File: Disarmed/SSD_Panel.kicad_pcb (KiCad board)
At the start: 2 copper layers, 181.6 x 193 mm, 15 parts, among them J1 Conn_02x04_Counter_Clockwise, U1 MAX7219, U2 MCP41010, U3 MAX7219, U4 MAX7219, U5 MAX7219

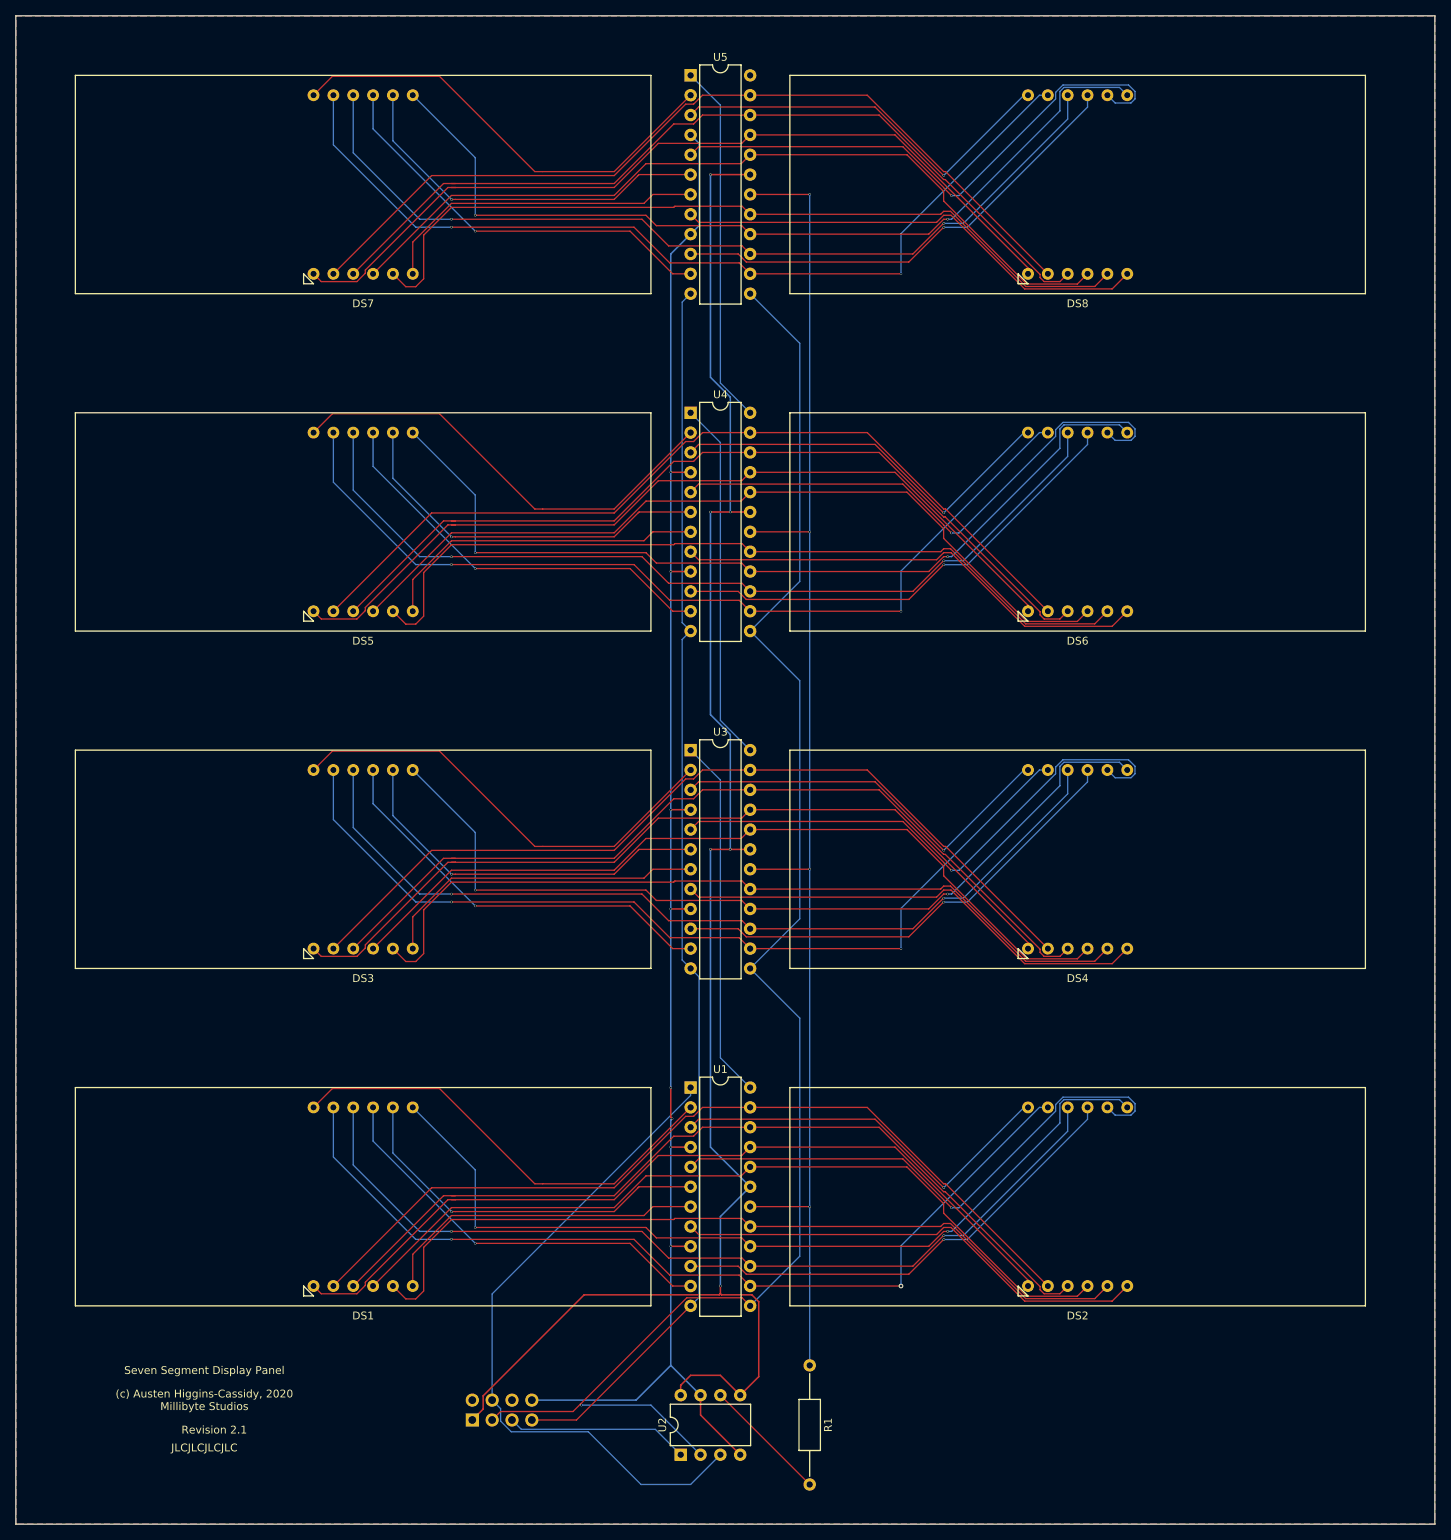
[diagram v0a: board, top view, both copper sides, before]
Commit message: Add new boards
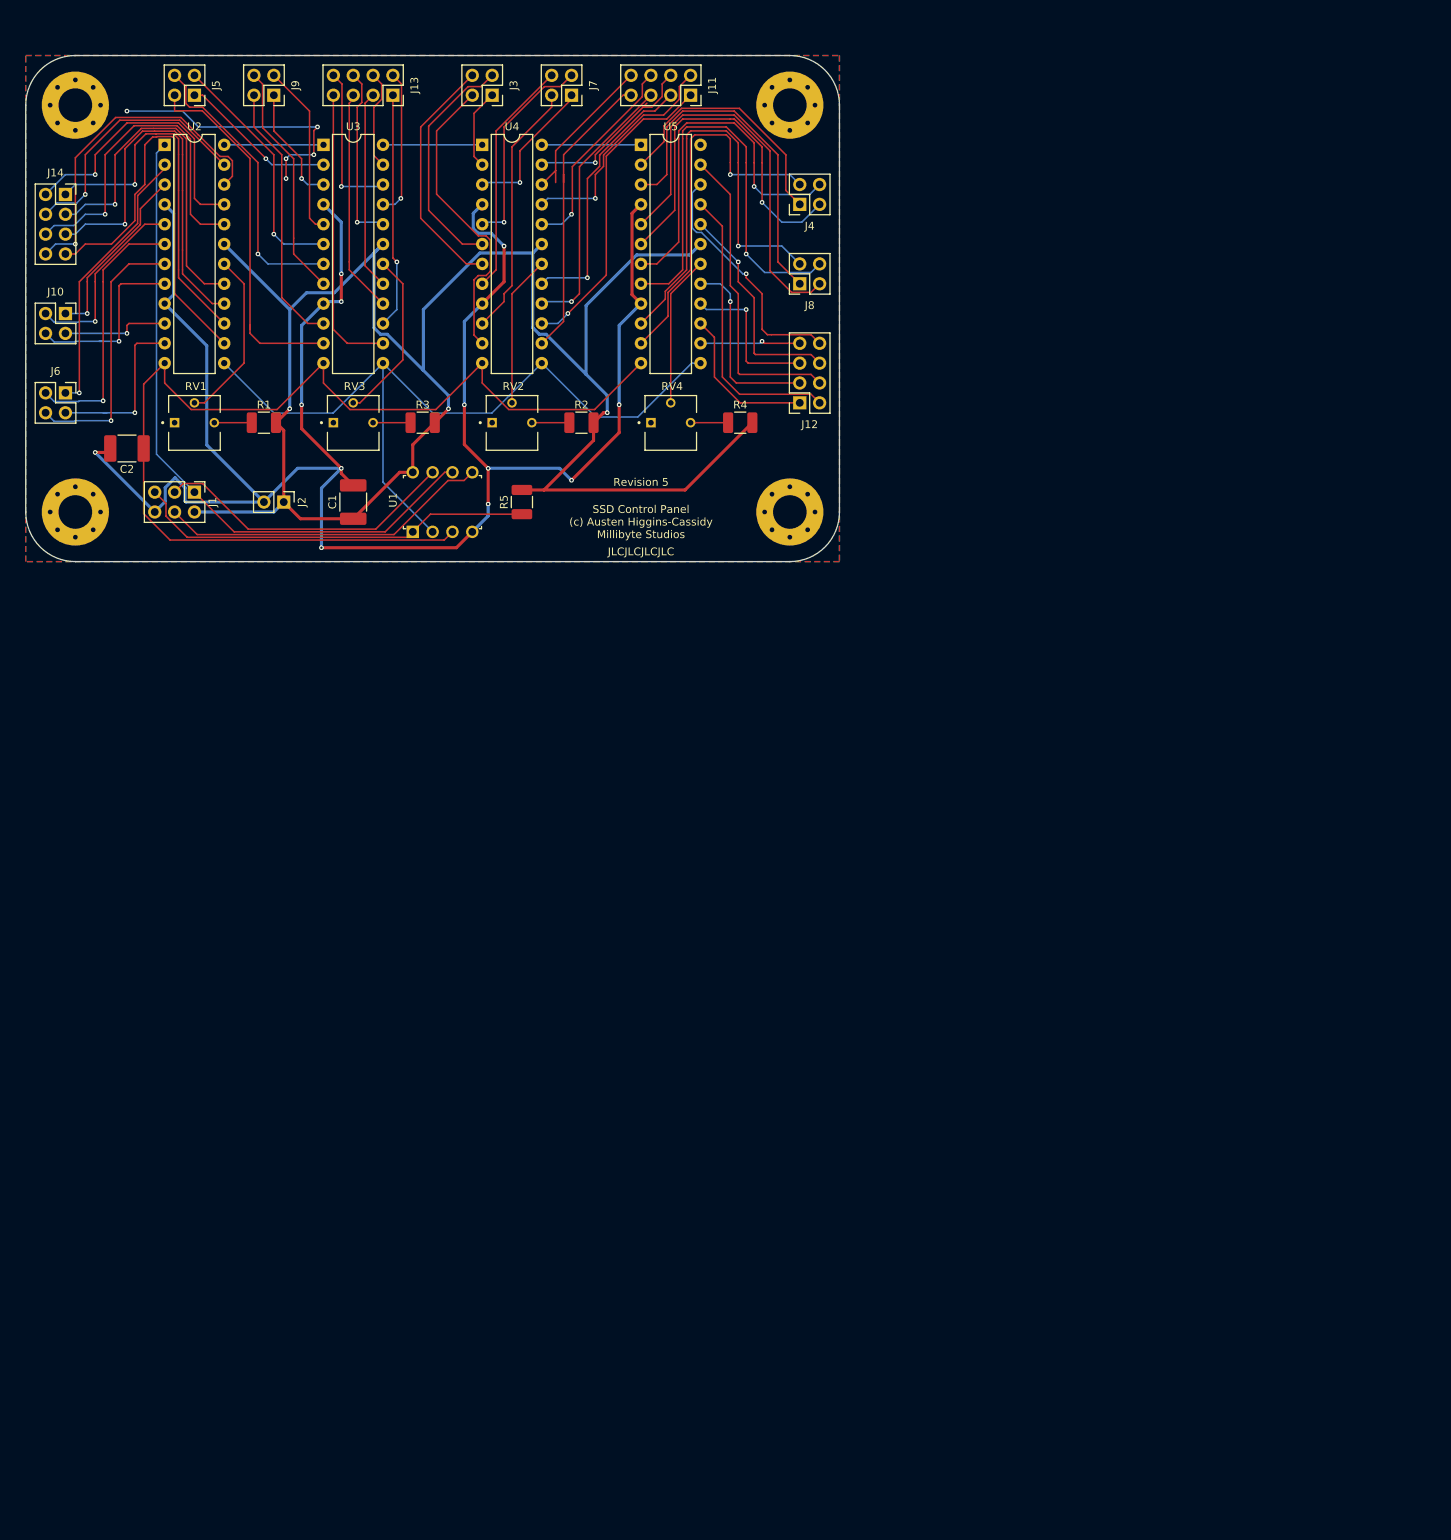
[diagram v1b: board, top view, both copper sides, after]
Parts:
- removed DS1, DS2, DS3, DS4, DS5, DS6, DS7, DS8: D8014CD, Disarmed:D8041CD
- added C1: 0.1uF, Capacitor_SMD:C_1812_4532Metric_Pad1.57x3.40mm_HandSolder, F.Cu at (57.1, 74.3)
- added C2: 10uF, Capacitor_SMD:C_1812_4532Metric_Pad1.57x3.40mm_HandSolder, F.Cu at (28.2, 67.4)
- added J10: Conn_02x02_Odd_Even, Connector_PinSocket_2.54mm:PinSocket_2x02_P2.54mm_Vertical, F.Cu at (20.3, 50.2)
- added J11: Conn_02x04_Odd_Even, Connector_PinSocket_2.54mm:PinSocket_2x04_P2.54mm_Vertical, F.Cu at (100.3, 22.2)
- added J12: Conn_02x04_Odd_Even, Connector_PinSocket_2.54mm:PinSocket_2x04_P2.54mm_Vertical, F.Cu at (114.3, 61.6)
- added J13: Conn_02x04_Odd_Even, Connector_PinSocket_2.54mm:PinSocket_2x04_P2.54mm_Vertical, F.Cu at (62.2, 22.2)
- added J14: Conn_02x04_Odd_Even, Connector_PinSocket_2.54mm:PinSocket_2x04_P2.54mm_Vertical, F.Cu at (20.3, 34.9)
- added J2: Conn_01x02_Male, Connector_PinHeader_2.54mm:PinHeader_1x02_P2.54mm_Vertical, F.Cu at (48.3, 74.3)
- added J3: Conn_02x02_Odd_Even, Connector_PinSocket_2.54mm:PinSocket_2x02_P2.54mm_Vertical, F.Cu at (74.9, 22.2)
- added J4: Conn_02x02_Odd_Even, Connector_PinSocket_2.54mm:PinSocket_2x02_P2.54mm_Vertical, F.Cu at (114.3, 36.2)
- added J5: Conn_02x02_Odd_Even, Connector_PinSocket_2.54mm:PinSocket_2x02_P2.54mm_Vertical, F.Cu at (36.8, 22.2)
- added J6: Conn_02x02_Odd_Even, Connector_PinSocket_2.54mm:PinSocket_2x02_P2.54mm_Vertical, F.Cu at (20.3, 60.3)
- added J7: Conn_02x02_Odd_Even, Connector_PinSocket_2.54mm:PinSocket_2x02_P2.54mm_Vertical, F.Cu at (85.1, 22.2)
- added J8: Conn_02x02_Odd_Even, Connector_PinSocket_2.54mm:PinSocket_2x02_P2.54mm_Vertical, F.Cu at (114.3, 46.4)
- added J9: Conn_02x02_Odd_Even, Connector_PinSocket_2.54mm:PinSocket_2x02_P2.54mm_Vertical, F.Cu at (47.0, 22.2)
- added R2: RMIN (2K), Resistor_SMD:R_1210_3225Metric_Pad1.30x2.65mm_HandSolder, F.Cu at (86.4, 64.1)
- added R3: RMIN (2K), Resistor_SMD:R_1210_3225Metric_Pad1.30x2.65mm_HandSolder, F.Cu at (66.0, 64.1)
- added R4: RMIN (2K), Resistor_SMD:R_1210_3225Metric_Pad1.30x2.65mm_HandSolder, F.Cu at (106.7, 64.1)
- added R5: 10K, Resistor_SMD:R_1210_3225Metric_Pad1.30x2.65mm_HandSolder, F.Cu at (78.7, 74.3)
- added REF**: MountingHole_4.3mm_M4_Pad_Via, Disarmed:MountingHole_4.3mm_M4_Pad_Via, F.Cu at (113.0, 23.5)
- added REF**: MountingHole_4.3mm_M4_Pad_Via, Disarmed:MountingHole_4.3mm_M4_Pad_Via, F.Cu at (113.0, 75.6)
- added REF**: MountingHole_4.3mm_M4_Pad_Via, Disarmed:MountingHole_4.3mm_M4_Pad_Via, F.Cu at (21.6, 75.6)
- added REF**: MountingHole_4.3mm_M4_Pad_Via, Disarmed:MountingHole_4.3mm_M4_Pad_Via, F.Cu at (21.6, 23.5)
- added RV1: R_POT, 3362P-1-103LF:TRIM_3362P-1-103LF, F.Cu at (36.8, 64.1)
- added RV2: R_POT, 3362P-1-103LF:TRIM_3362P-1-103LF, F.Cu at (77.5, 64.1)
- added RV3: R_POT, 3362P-1-103LF:TRIM_3362P-1-103LF, F.Cu at (57.1, 64.1)
- added RV4: R_POT, 3362P-1-103LF:TRIM_3362P-1-103LF, F.Cu at (97.8, 64.1)
- J1: value Conn_02x04_Counter_Clockwise -> Conn_02x03_Odd_Even; footprint Connector_PinSocket_2.54mm:PinSocket_2x04_P2.54mm_Vertical -> Connector_PinHeader_2.54mm:PinHeader_2x03_P2.54mm_Vertical; moved to F.Cu
- R1: value 2k -> RMIN (2K); footprint Resistor_THT:R_Axial_DIN0207_L6.3mm_D2.5mm_P15.24mm_Horizontal -> Resistor_SMD:R_1210_3225Metric_Pad1.30x2.65mm_HandSolder
- U1: value MAX7219 -> ATTINY85-20PU; footprint Package_DIP:DIP-24_W7.62mm -> digikey-footprints:DIP-8_W7.62mm
- U2: value MCP41010 -> MAX7219; footprint Package_DIP:DIP-8_W7.62mm -> Package_DIP:DIP-24_W7.62mm
- moved U2 180.2 mm to (33.0, 28.6), turned to 0 degrees
- moved R1 139.4 mm to (45.7, 64.1), turned to 0 degrees
- moved J1 124.0 mm to (36.8, 73.0)
- moved U3 90.6 mm to (53.3, 28.6)
- moved U1 79.5 mm to (64.8, 78.1), turned to 90 degrees
- moved U4 43.4 mm to (73.7, 28.6)
- moved U5 10.9 mm to (94.0, 28.6)
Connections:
- J1 pad 1: /SSD_Panel/VCC -> /MISO_DATA
- J1 pad 2: Net-(J1-Pad2) -> +5V
- J1 pad 3: /SSD_Panel/CLK -> /SCK_SCL
- J1 pad 4: /SSD_Panel/DATA -> /MOSI_SDA
- J1 pad 5: /SSD_Panel/CCSEL -> /RST
- J1 pad 6: Net-(J1-Pad6) -> GND
- R1 pad 1: /SSD_Panel/ISET -> Net-(R1-Pad1)
- R1 pad 2: Net-(R1-Pad2) -> +5V
- U1 pad 1: /SSD_Panel/DATA -> /RST
- U1 pad 2: /SSD_Panel/DIG0 -> /CLK
- U1 pad 3: /SSD_Panel/DIG4 -> /LOAD
- U1 pad 4: /SSD_Panel/GND -> GND
- U1 pad 5: /SSD_Panel/DIG6 -> /MOSI_SDA
- U1 pad 6: /SSD_Panel/DIG2 -> /MISO_DATA
- U1 pad 7: /SSD_Panel/DIG3 -> /SCK_SCL
- U1 pad 8: /SSD_Panel/DIG7 -> +5V
- U2 pad 1: /SSD_Panel/CCSEL -> /MISO_DATA
- U2 pad 2: /SSD_Panel/CLK -> /DIG0
- U2 pad 3: /SSD_Panel/DATA -> /DIG4
- U2 pad 4: /SSD_Panel/GND -> GND
- U2 pad 5: /SSD_Panel/VCC -> /DIG6
- U2 pad 6: Net-(R1-Pad2) -> /DIG2
- U2 pad 7: /SSD_Panel/GND -> /DIG3
- U2 pad 8: /SSD_Panel/VCC -> /DIG7
- U3 pad 1: Net-(U1-Pad24) -> Net-(U2-Pad24)
- U3 pad 10: /SSD_Panel/DIG13 -> /DIG13
- U3 pad 11: /SSD_Panel/DIG9 -> /DIG9
- U3 pad 12: /SSD_Panel/LOAD -> /LOAD
- U3 pad 13: /SSD_Panel/CLK -> /CLK
- U3 pad 14: /SSD_Panel/A2 -> /A2
- U3 pad 15: /SSD_Panel/F2 -> /F2
- U3 pad 16: /SSD_Panel/B2 -> /B2
- U3 pad 17: /SSD_Panel/G2 -> /G2
- U3 pad 18: /SSD_Panel/ISET -> /ISET2
- U3 pad 19: /SSD_Panel/VCC -> +5V
- U3 pad 2: /SSD_Panel/DIG8 -> /DIG8
- U3 pad 20: /SSD_Panel/C2 -> /C2
- U3 pad 21: /SSD_Panel/E2 -> /E2
- U3 pad 22: /SSD_Panel/DP2 -> /DP2
- U3 pad 23: /SSD_Panel/D2 -> /D2
- U3 pad 3: /SSD_Panel/DIG12 -> /DIG12
- U3 pad 4: /SSD_Panel/GND -> GND
- U3 pad 5: /SSD_Panel/DIG14 -> /DIG14
- U3 pad 6: /SSD_Panel/DIG10 -> /DIG10
- U3 pad 7: /SSD_Panel/DIG11 -> /DIG11
- U3 pad 8: /SSD_Panel/DIG15 -> /DIG15
- U3 pad 9: /SSD_Panel/GND -> GND
- U4 pad 10: /SSD_Panel/DIG21 -> /DIG21
- U4 pad 11: /SSD_Panel/DIG17 -> /DIG17
- U4 pad 12: /SSD_Panel/LOAD -> /LOAD
- U4 pad 13: /SSD_Panel/CLK -> /CLK
- U4 pad 14: /SSD_Panel/A3 -> /A3
- U4 pad 15: /SSD_Panel/F3 -> /F3
- U4 pad 16: /SSD_Panel/B3 -> /B3
- U4 pad 17: /SSD_Panel/G3 -> /G3
- U4 pad 18: /SSD_Panel/ISET -> /ISET3
- U4 pad 19: /SSD_Panel/VCC -> +5V
- U4 pad 2: /SSD_Panel/DIG16 -> /DIG16
- U4 pad 20: /SSD_Panel/C3 -> /C3
- U4 pad 21: /SSD_Panel/E3 -> /E3
- U4 pad 22: /SSD_Panel/DP3 -> /DP3
- U4 pad 23: /SSD_Panel/D3 -> /D3
- U4 pad 3: /SSD_Panel/DIG20 -> /DIG20
- U4 pad 4: /SSD_Panel/GND -> GND
- U4 pad 5: /SSD_Panel/DIG22 -> /DIG22
- U4 pad 6: /SSD_Panel/DIG18 -> /DIG18
- U4 pad 7: /SSD_Panel/DIG19 -> /DIG19
- U4 pad 8: /SSD_Panel/DIG23 -> /DIG23
- U4 pad 9: /SSD_Panel/GND -> GND
- U5 pad 10: /SSD_Panel/DIG29 -> /DIG29
- U5 pad 11: /SSD_Panel/DIG25 -> /DIG25
- U5 pad 12: /SSD_Panel/LOAD -> /LOAD
- U5 pad 13: /SSD_Panel/CLK -> /CLK
- U5 pad 14: /SSD_Panel/A4 -> /A4
- U5 pad 15: /SSD_Panel/F4 -> /F4
- U5 pad 16: /SSD_Panel/B4 -> /B4
- U5 pad 17: /SSD_Panel/G4 -> /G4
- U5 pad 18: /SSD_Panel/ISET -> /ISET4
- U5 pad 19: /SSD_Panel/VCC -> +5V
- U5 pad 2: /SSD_Panel/DIG24 -> /DIG24
- U5 pad 20: /SSD_Panel/C4 -> /C4
- U5 pad 21: /SSD_Panel/E4 -> /E4
- U5 pad 22: /SSD_Panel/DP4 -> /DP4
- U5 pad 23: /SSD_Panel/D4 -> /D4
- U5 pad 24: Net-(U5-Pad24) -> (no net)
- U5 pad 3: /SSD_Panel/DIG28 -> /DIG28
- U5 pad 4: /SSD_Panel/GND -> GND
- U5 pad 5: /SSD_Panel/DIG30 -> /DIG30
- U5 pad 6: /SSD_Panel/DIG26 -> /DIG26
- U5 pad 7: /SSD_Panel/DIG27 -> /DIG27
- U5 pad 8: /SSD_Panel/DIG31 -> /DIG31
- U5 pad 9: /SSD_Panel/GND -> GND
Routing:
- net GND: track 0.00 -> 262.8 mm, vias 0 -> 12
- net +5V: track 0.00 -> 245.5 mm, vias 0 -> 3
- net /SSD_Panel/VCC: track 232.4 -> 0.00 mm, vias 6 -> 0
- net /SSD_Panel/GND: track 210.2 -> 0.00 mm, vias 8 -> 0
- net /SSD_Panel/CLK: track 203.3 -> 0.00 mm, vias 1 -> 0
- net /SSD_Panel/ISET: track 180.5 -> 0.00 mm, vias 4 -> 0
- net /SSD_Panel/LOAD: track 158.6 -> 0.00 mm
- net /LOAD: track 0.00 -> 141.9 mm
- net /SSD_Panel/A1: track 117.1 -> 0.00 mm, vias 2 -> 0
- net /SSD_Panel/A4: track 117.1 -> 0.00 mm, vias 2 -> 0
- net /SSD_Panel/A3: track 117.1 -> 0.00 mm, vias 2 -> 0
- net /SSD_Panel/A2: track 117.1 -> 0.00 mm, vias 2 -> 0
- net /SSD_Panel/F1: track 114.4 -> 0.00 mm, vias 2 -> 0
- net /SSD_Panel/F4: track 114.4 -> 0.00 mm, vias 2 -> 0
- net /SSD_Panel/F3: track 114.4 -> 0.00 mm, vias 2 -> 0
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- added copper zone on B.Cu, net GND
- added copper zone on F.Cu, net GND
- removed copper zone on B.Cu, net /SSD_Panel/GND
- removed copper zone on F.Cu, net /SSD_Panel/GND
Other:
- board size 181.6 x 193 mm -> 104.1 x 64.8 mm
- net class Default: clearance 0.1524 -> 0.15; trace_width 0.16 -> 0.2
- net class Power: clearance 0.2 -> 0.15; trace_width 0.2 -> 0.4
- rule trace_clearance: 0.1524 -> 0.15
- board text added: "Revision 5"
- board text added: "SSD Control Panel (c) Austen Higgins-Cassidy Millibyte Studios"
- board text removed: "(c) Austen Higgins-Cassidy, 2020 Millibyte Studios"
- board text removed: "Revision 2.1"
- board text removed: "Seven Segment Display Panel"
